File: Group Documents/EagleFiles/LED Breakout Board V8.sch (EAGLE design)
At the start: 6 parts

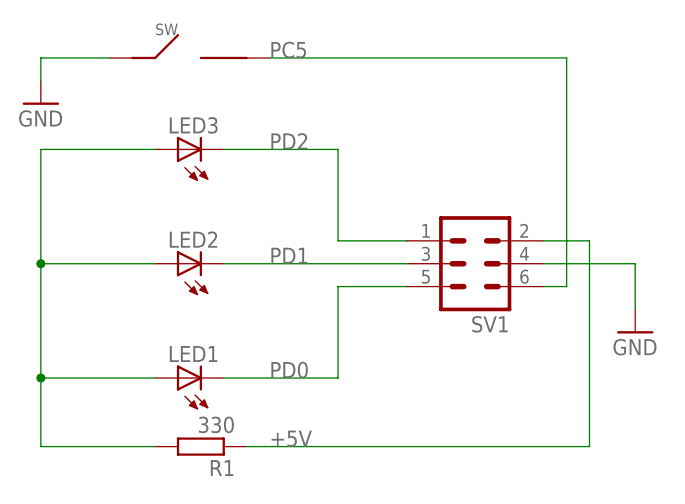
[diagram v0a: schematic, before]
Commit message: LED BOB
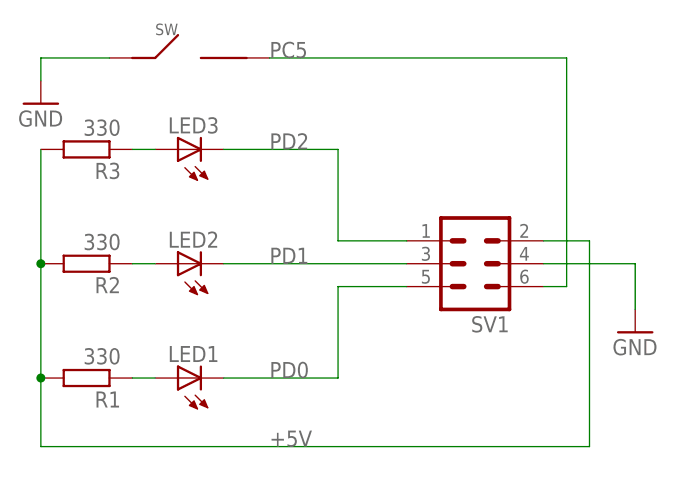
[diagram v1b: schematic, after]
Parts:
- added R2, R3: 330, eagle-ltspice:R0207/10
- R1: device eagle-ltspice:R0204/7 -> eagle-ltspice:R0207/10
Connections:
- removed net N$1: LED1.A, LED2.A, LED3.A, R1.2
- new net N$2: LED3.A, R3.1
- new net N$3: LED2.A, R2.1
- new net N$4: LED1.A, R1.1
- net +5V: now also R1.2, R2.2, R3.2; no longer R1.1
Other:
- moved on the sheet: R1
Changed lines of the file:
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@@
 <part name="LED3" library="led" deviceset="LED" device="10MM"/>
 <part name="GND2" library="supply1" deviceset="GND" device=""/>
-<part name="R1" library="eagle-ltspice" deviceset="R" device="0204/7" value="330"/>
+<part name="R2" library="eagle-ltspice" deviceset="R" device="0207/10" value="330"/>
+<part name="R3" library="eagle-ltspice" deviceset="R" device="0207/10" value="330"/>
+<part name="R1" library="eagle-ltspice" deviceset="R" device="0207/10" value="330"/>
 </parts>
 <sheets>
@@
 <instance part="LED3" gate="G$1" x="83.82" y="76.2" rot="R90"/>
 <instance part="GND2" gate="1" x="68.58" y="81.28"/>
-<instance part="R1" gate="G$1" x="86.36" y="43.18" rot="R180"/>
+<instance part="R2" gate="G$1" x="73.66" y="63.5" rot="R180"/>
+<instance part="R3" gate="G$1" x="73.66" y="76.2" rot="R180"/>
+<instance part="R1" gate="G$1" x="73.66" y="50.8" rot="R180"/>
 </instances>
 <busses>
@@
 <wire x1="124.46" y1="66.04" x2="129.54" y2="66.04" width="0.1524" layer="91"/>
 <wire x1="129.54" y1="66.04" x2="129.54" y2="43.18" width="0.1524" layer="91"/>
-<wire x1="91.44" y1="43.18" x2="129.54" y2="43.18" width="0.1524" layer="91"/>
 <label x="93.98" y="43.18" size="1.778" layer="95"/>
-<pinref part="R1" gate="G$1" pin="1"/>
+<pinref part="R2" gate="G$1" pin="2"/>
+<wire x1="68.58" y1="50.8" x2="68.58" y2="63.5" width="0.1524" layer="91"/>
+<wire x1="68.58" y1="63.5" x2="68.58" y2="76.2" width="0.1524" layer="91"/>
+<junction x="68.58" y="63.5"/>
+<pinref part="R3" gate="G$1" pin="2"/>
+<pinref part="R1" gate="G$1" pin="2"/>
+<wire x1="129.54" y1="43.18" x2="68.58" y2="43.18" width="0.1524" layer="91"/>
+<wire x1="68.58" y1="43.18" x2="68.58" y2="50.8" width="0.1524" layer="91"/>
+<junction x="68.58" y="50.8"/>
 </segment>
 </net>
-<net name="N$1" class="0">
+<net name="N$2" class="0">
 <segment>
-<wire x1="81.28" y1="43.18" x2="68.58" y2="43.18" width="0.1524" layer="91"/>
-<wire x1="68.58" y1="43.18" x2="68.58" y2="50.8" width="0.1524" layer="91"/>
-<wire x1="68.58" y1="50.8" x2="68.58" y2="63.5" width="0.1524" layer="91"/>
-<wire x1="68.58" y1="63.5" x2="68.58" y2="76.2" width="0.1524" layer="91"/>
-<wire x1="68.58" y1="76.2" x2="81.28" y2="76.2" width="0.1524" layer="91"/>
-<wire x1="68.58" y1="63.5" x2="81.28" y2="63.5" width="0.1524" layer="91"/>
-<junction x="68.58" y="63.5"/>
-<wire x1="68.58" y1="50.8" x2="81.28" y2="50.8" width="0.1524" layer="91"/>
-<junction x="68.58" y="50.8"/>
-<pinref part="LED1" gate="G$1" pin="A"/>
-<pinref part="LED2" gate="G$1" pin="A"/>
+<pinref part="R3" gate="G$1" pin="1"/>
 <pinref part="LED3" gate="G$1" pin="A"/>
-<pinref part="R1" gate="G$1" pin="2"/>
+<wire x1="78.74" y1="76.2" x2="81.28" y2="76.2" width="0.1524" layer="91"/>
 </segment>
 </net>
+<net name="N$3" class="0">
+<segment>
+<pinref part="R2" gate="G$1" pin="1"/>
+<pinref part="LED2" gate="G$1" pin="A"/>
+<wire x1="78.74" y1="63.5" x2="81.28" y2="63.5" width="0.1524" layer="91"/>
+</segment>
+</net>
+<net name="N$4" class="0">
+<segment>
+<pinref part="R1" gate="G$1" pin="1"/>
+<pinref part="LED1" gate="G$1" pin="A"/>
+<wire x1="78.74" y1="50.8" x2="81.28" y2="50.8" width="0.1524" layer="91"/>
+</segment>
+</net>
